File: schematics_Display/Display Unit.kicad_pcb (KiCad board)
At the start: 2 copper layers, 108.5 x 43.5 mm, 7 parts, among them M1 Stepper_Motor_bipolar, SW1 SW_Push, U2 XIAO_ESP32C3

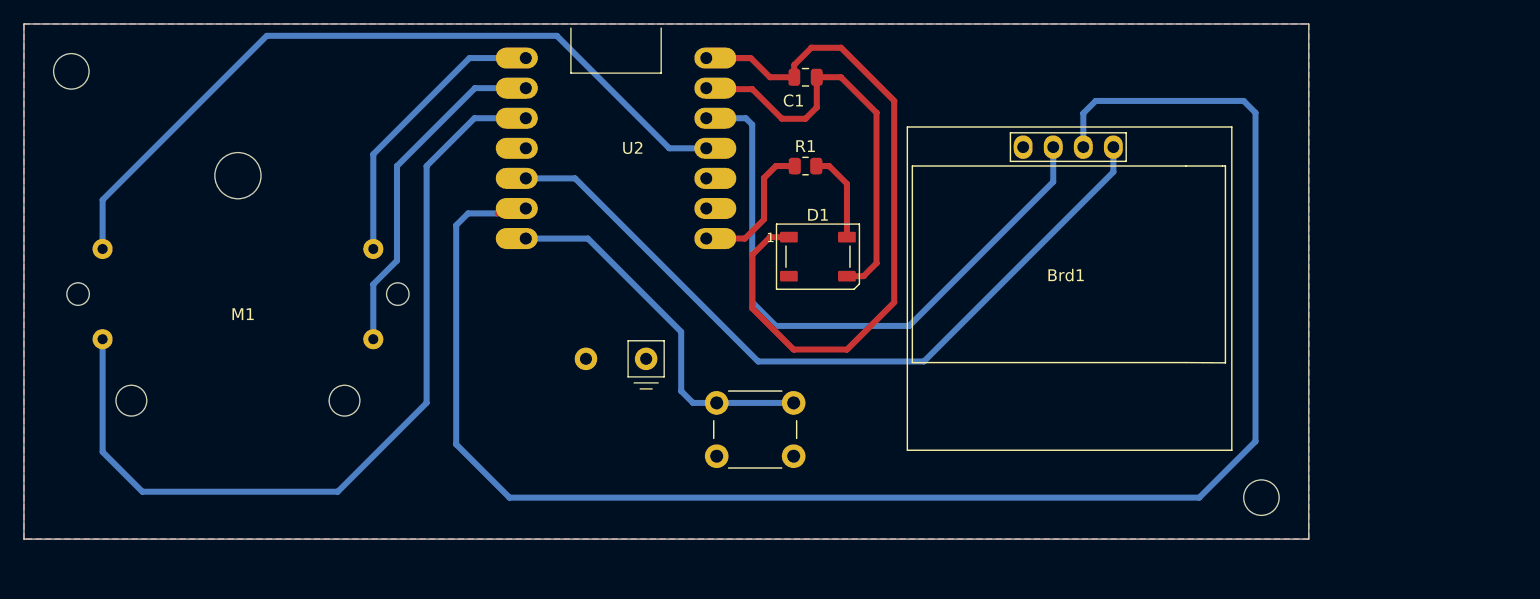
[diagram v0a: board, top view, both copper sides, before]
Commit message: add coding, pcb, and revised sketches
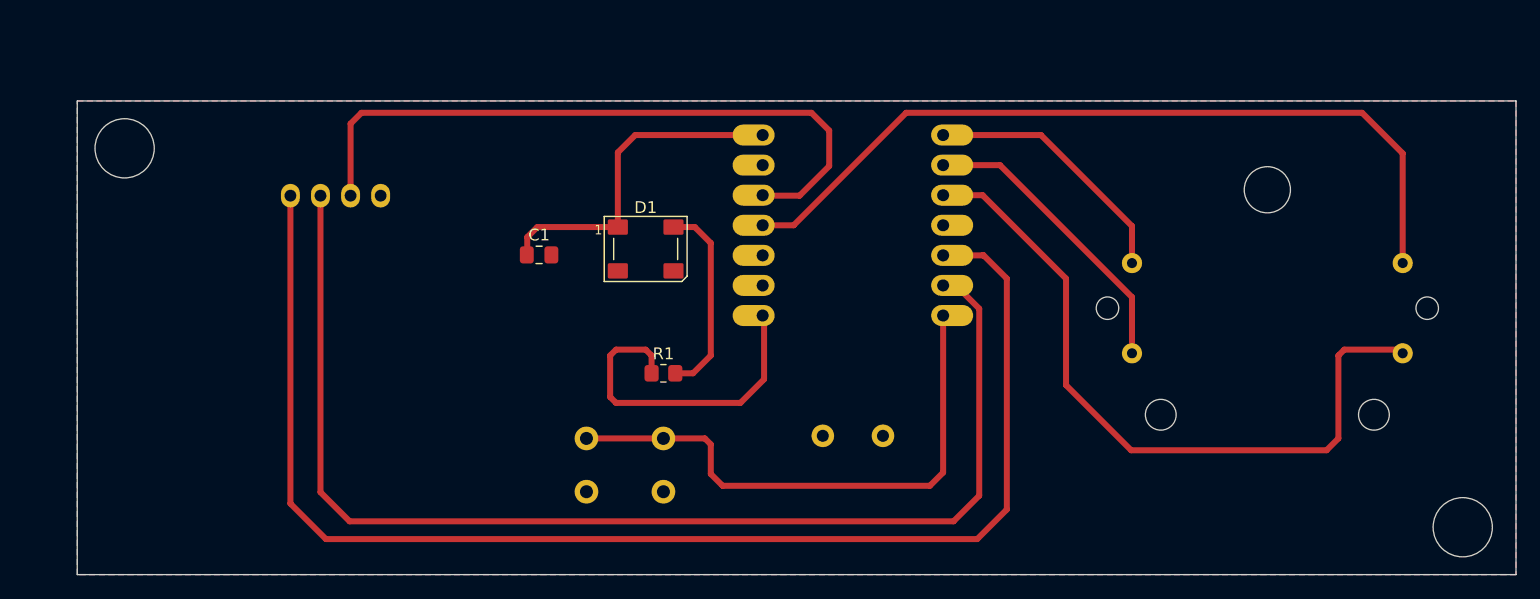
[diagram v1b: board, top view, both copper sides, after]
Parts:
- Brd1, M1, SW1, U2: moved to B.Cu
- C1: footprint Capacitor_SMD:C_0805_2012Metric -> Capacitor_SMD:C_0805_2012Metric_Pad1.18x1.45mm_HandSolder
- R1: footprint Resistor_SMD:R_0805_2012Metric -> Resistor_SMD:R_0805_2012Metric_Pad1.20x1.40mm_HandSolder
- moved M1 81.9 mm to (182.0, 80.7), turned to 180 degrees
- moved Brd1 61.6 mm to (106.0, 71.6), turned to 180 degrees
- moved C1 27.0 mm to (123.0, 66.0)
- moved R1 21.2 mm to (133.5, 76.0)
- moved U2 21.0 mm to (149.5, 63.5), turned to 180 degrees
- moved D1 14.6 mm to (132.0, 65.5)
- moved SW1 5.41 mm to (133.5, 81.5), turned to 180 degrees
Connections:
- C1 pad 2: Net-(D1-VSS) -> GND
- D1 pad 3: Net-(D1-VSS) -> GND
- U2 pad 13: Net-(D1-VSS) -> GND
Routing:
- net Net-(Brd1-SDA): track 64.8 -> 114.5 mm
- net Net-(Brd1-SCL): track 142.3 -> 102.2 mm
- net Net-(D1-VSS): track 35.4 -> 0.00 mm
- net Net-(D1-VDD): track 60.4 -> 28.7 mm
- net Net-(U2-GPIO44_D7_RX): track 12.1 -> 28.4 mm
- net Net-(U2-GPIO43_TX_D6): track 31.3 -> 47.0 mm
- net Net-(U2-GPIO3_A2_D2): track 72.8 -> 60.8 mm
- net Net-(D1-DIN): track 7.71 -> 16.8 mm
- net Net-(U2-GPIO9_A10_D10_COPI): track 64.8 -> 68.7 mm
- net Net-(M1--): track 29.1 -> 25.3 mm
- net Net-(Brd1-VCC): track 54.4 -> 57.2 mm
- net Net-(U2-GPIO1_A0_D0): track 24.2 -> 22.3 mm
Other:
- board size 108.5 x 43.5 mm -> 121.5 x 40 mm
